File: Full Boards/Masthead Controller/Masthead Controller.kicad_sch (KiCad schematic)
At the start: 165 parts, among them Q1 2N7002, Q2 2N7002, SW1 SW_MEC_5G, SW2 SW_MEC_5G

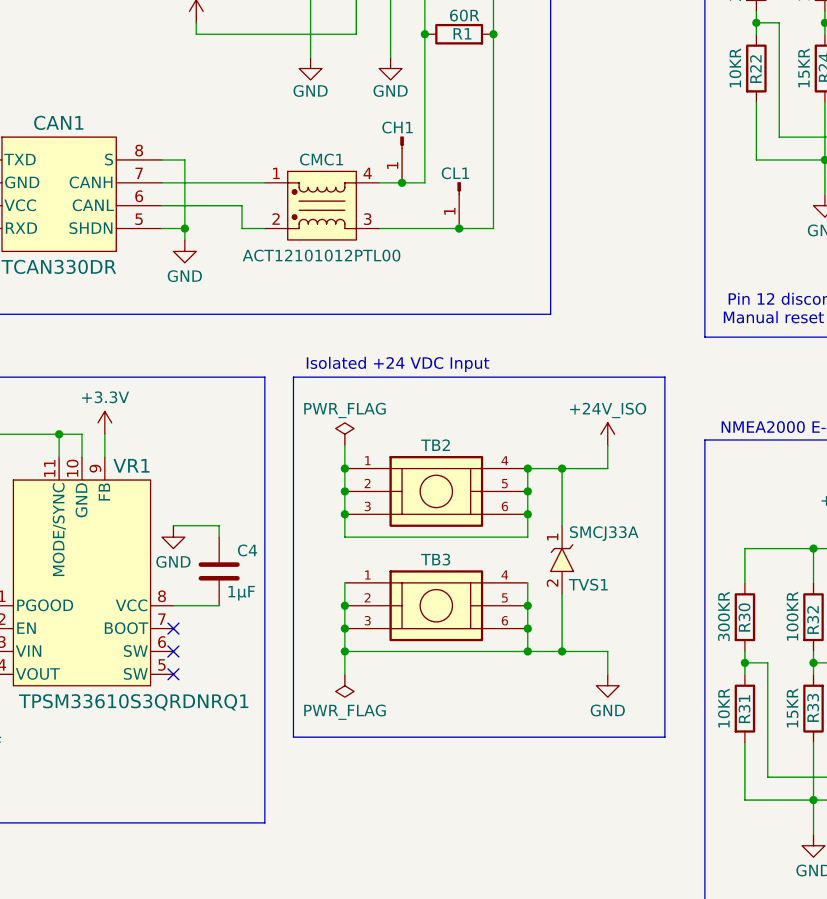
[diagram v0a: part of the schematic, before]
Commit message: Updated schematic and PCB to use the updated symbols and footprints.
Signed-off-by: digimer <digital.mermaid@gmail.com>
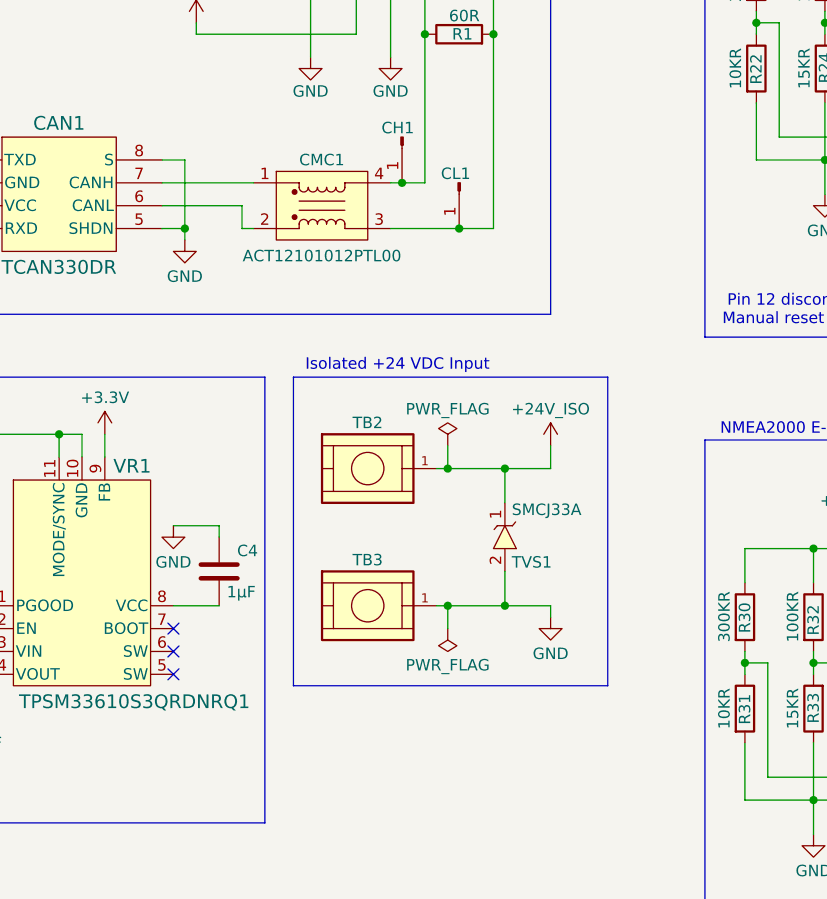
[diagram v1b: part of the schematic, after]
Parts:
- CMC1: Part (none) -> TDK ACT12101012PTL00
- TB2, TB3: value Keystone Electronics 7799 -> 7799; Part (none) -> Keystone 7799
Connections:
- net +24V_ISO: no longer TB2.2, TB2.3, TB2.4, TB2.5, TB2.6
- net GND: no longer TB3.2, TB3.3, TB3.4, TB3.5, TB3.6
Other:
- moved on the sheet: TVS1
